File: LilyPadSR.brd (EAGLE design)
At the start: 50.9 x 50.9 mm, 40 parts, among them IC1 74HC595D, IC2 74HC595D

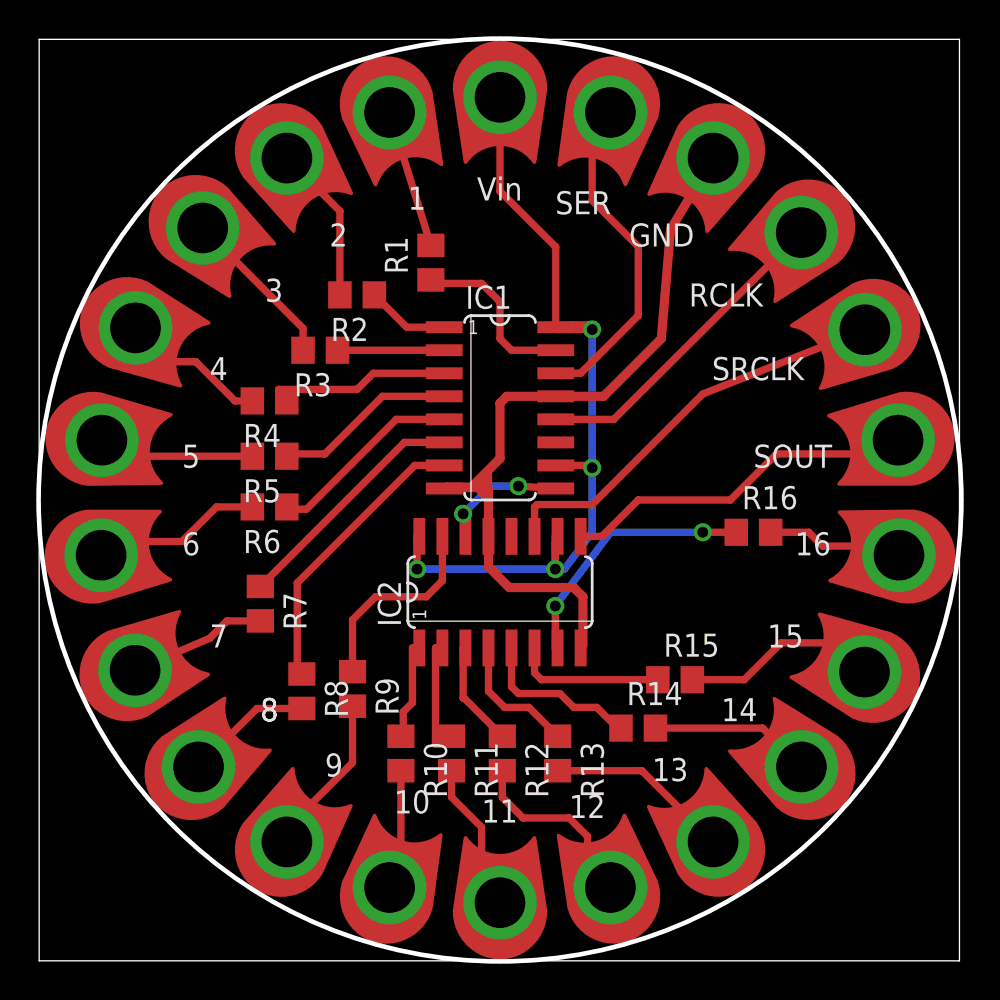
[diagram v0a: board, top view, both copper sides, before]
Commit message: new design outputted and gerber generated
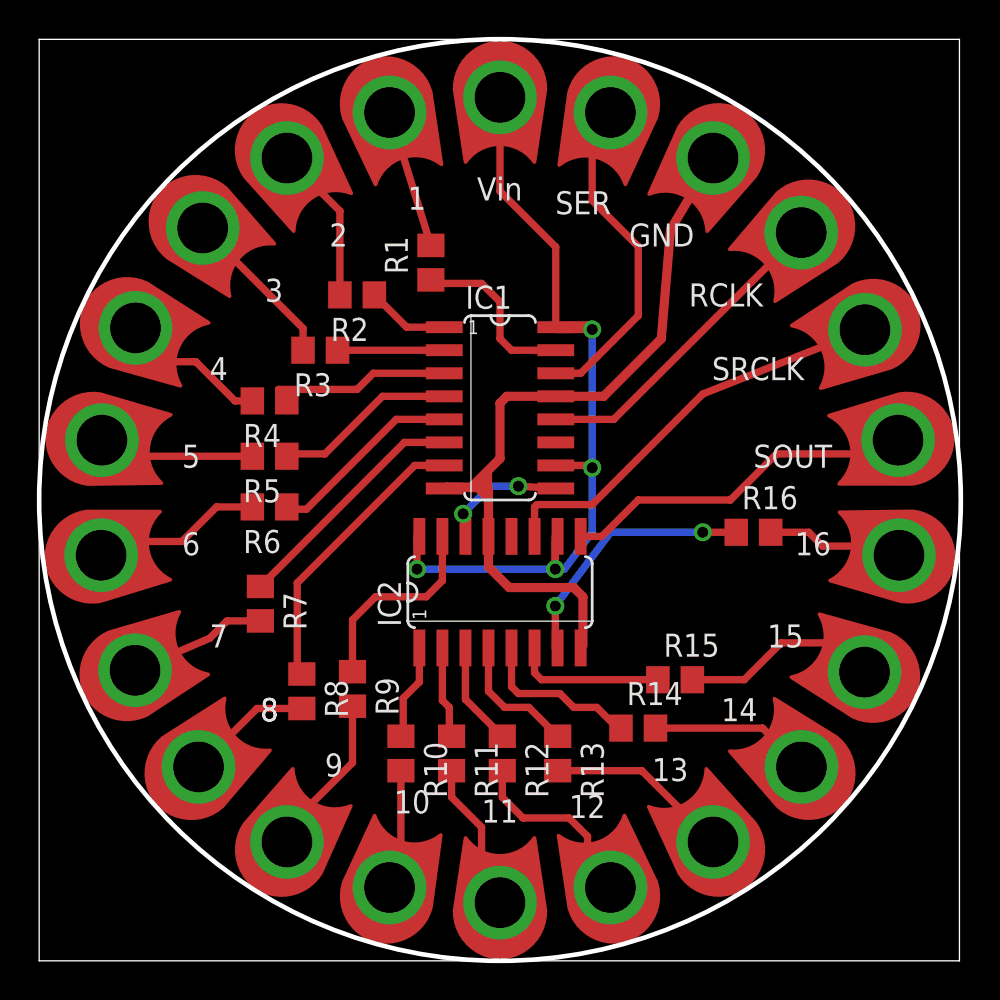
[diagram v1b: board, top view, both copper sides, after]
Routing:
- net N$11: track 7.02 -> 5.08 mm
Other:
- board size 50.9 x 50.9 mm -> 50.8 x 50.8 mm
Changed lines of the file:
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@@
 <wire x1="50.724" y1="80" x2="0" y2="80" width="0" layer="20"/>
 <wire x1="0" y1="80" x2="0" y2="29.21" width="0" layer="20"/>
-<circle x="25.4" y="54.61" radius="25.431728125" width="0.254" layer="20"/>
+<circle x="25.4" y="54.61" radius="25.4" width="0.254" layer="20"/>
 <rectangle x1="24.13" y1="55.372" x2="24.892" y2="55.88" layer="1"/>
 <rectangle x1="24.384" y1="55.118" x2="24.765" y2="56.1594" layer="1"/>
@@
 <contactref element="IC2" pad="1"/>
 <contactref element="R10" pad="1"/>
-<wire x1="20.955" y1="46.4566" x2="20.574" y2="46.4566" width="0.4064" layer="1"/>
-<wire x1="20.574" y1="46.4566" x2="20.574" y2="43.434" width="0.4064" layer="1"/>
-<wire x1="20.574" y1="43.434" x2="20.066" y2="42.926" width="0.4064" layer="1"/>
-<wire x1="20.066" y1="42.926" x2="20.066" y2="41.7169875" width="0.4064" layer="1"/>
+<wire x1="20.955" y1="46.4566" x2="20.955" y2="44.577" width="0.4064" layer="1"/>
+<wire x1="20.955" y1="44.577" x2="20.066" y2="43.688" width="0.4064" layer="1"/>
+<wire x1="20.066" y1="43.688" x2="20.066" y2="41.7169875" width="0.4064" layer="1"/>
 <wire x1="20.066" y1="41.7169875" x2="19.9390125" y2="41.59" width="0.4064" layer="1"/>
 </signal>
@@
 <contactref element="IC2" pad="2"/>
 <contactref element="R11" pad="1"/>
-<wire x1="22.225" y1="46.4566" x2="21.844" y2="46.4566" width="0.4064" layer="1"/>
-<wire x1="21.844" y1="46.4566" x2="21.844" y2="41.148" width="0.4064" layer="1"/>
-<wire x1="21.844" y1="41.148" x2="22.7312375" y2="41.148" width="0.4064" layer="1"/>
-<wire x1="22.7312375" y1="41.148" x2="22.7312375" y2="41.59" width="0.4064" layer="1"/>
+<wire x1="22.225" y1="46.4566" x2="22.225" y2="43.561" width="0.4064" layer="1"/>
+<wire x1="22.225" y1="43.561" x2="22.606" y2="43.18" width="0.4064" layer="1"/>
+<wire x1="22.606" y1="43.18" x2="22.606" y2="41.7152375" width="0.4064" layer="1"/>
+<wire x1="22.606" y1="41.7152375" x2="22.7312375" y2="41.59" width="0.4064" layer="1"/>
 </signal>
 <signal name="N$12">
 <contactref element="IC2" pad="3"/>
 <contactref element="R12" pad="1"/>
-<wire x1="23.495" y1="46.4566" x2="23.368" y2="46.4566" width="0.4064" layer="1"/>
-<wire x1="23.368" y1="46.4566" x2="23.368" y2="43.688" width="0.4064" layer="1"/>
-<wire x1="23.368" y1="43.688" x2="23.42830625" y2="43.688" width="0.4064" layer="1"/>
-<wire x1="23.42830625" y1="43.688" x2="25.52630625" y2="41.59" width="0.4064" layer="1"/>
+<wire x1="23.495" y1="46.4566" x2="23.495" y2="43.62130625" width="0.4064" layer="1"/>
+<wire x1="23.495" y1="43.62130625" x2="25.52630625" y2="41.59" width="0.4064" layer="1"/>
 </signal>
 <signal name="N$13">
